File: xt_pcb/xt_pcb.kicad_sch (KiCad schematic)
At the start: 20 parts, among them J1 Conn_01x04_Socket, J2 USB_C_Receptacle_USB2.0_16P, U1 AMS1117-3.3, U2 ATmega32U4-A, U3 USB6B1, Y1 Crystal_GND24_Small

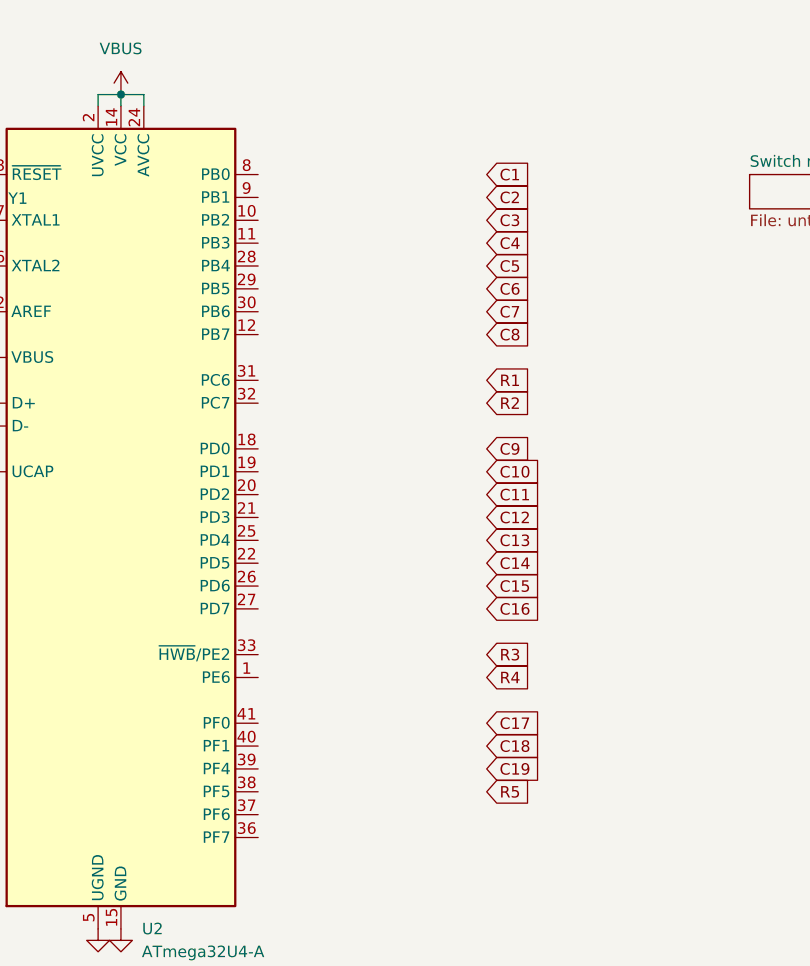
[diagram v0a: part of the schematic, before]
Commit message: tracing finished
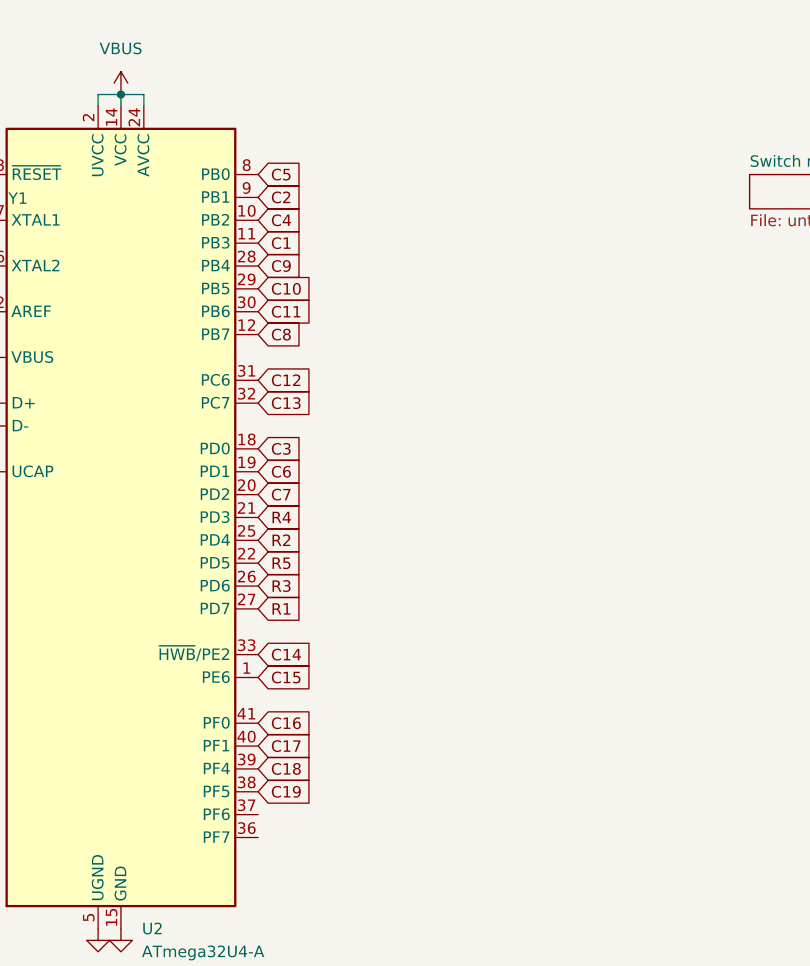
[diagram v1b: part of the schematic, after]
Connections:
- net C1: now also U2.11 (PB3)
- net C10: now also U2.29 (PB5)
- net C11: now also U2.30 (PB6)
- net C12: now also U2.31 (PC6)
- net C13: now also U2.32 (PC7)
- net C14: now also U2.33 (~{HWB}/PE2)
- net C15: now also U2.1 (PE6)
- net C16: now also U2.41 (PF0)
- net C17: now also U2.40 (PF1)
- net C18: now also U2.39 (PF4)
- net C19: now also U2.38 (PF5)
- net C2: now also U2.9 (PB1)
- net C3: now also U2.18 (PD0)
- net C4: now also U2.10 (PB2)
- net C5: now also U2.8 (PB0)
- net C6: now also U2.19 (PD1)
- net C7: now also U2.20 (PD2)
- net C8: now also U2.12 (PB7)
- net C9: now also U2.28 (PB4)
- net R1: now also U2.27 (PD7)
- net R2: now also U2.25 (PD4)
- net R3: now also U2.26 (PD6)
- net R4: now also U2.21 (PD3)
- net R5: now also U2.22 (PD5)
